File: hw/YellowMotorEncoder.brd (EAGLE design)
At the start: 35 x 22.2 mm, 20 parts, among them P1 M1

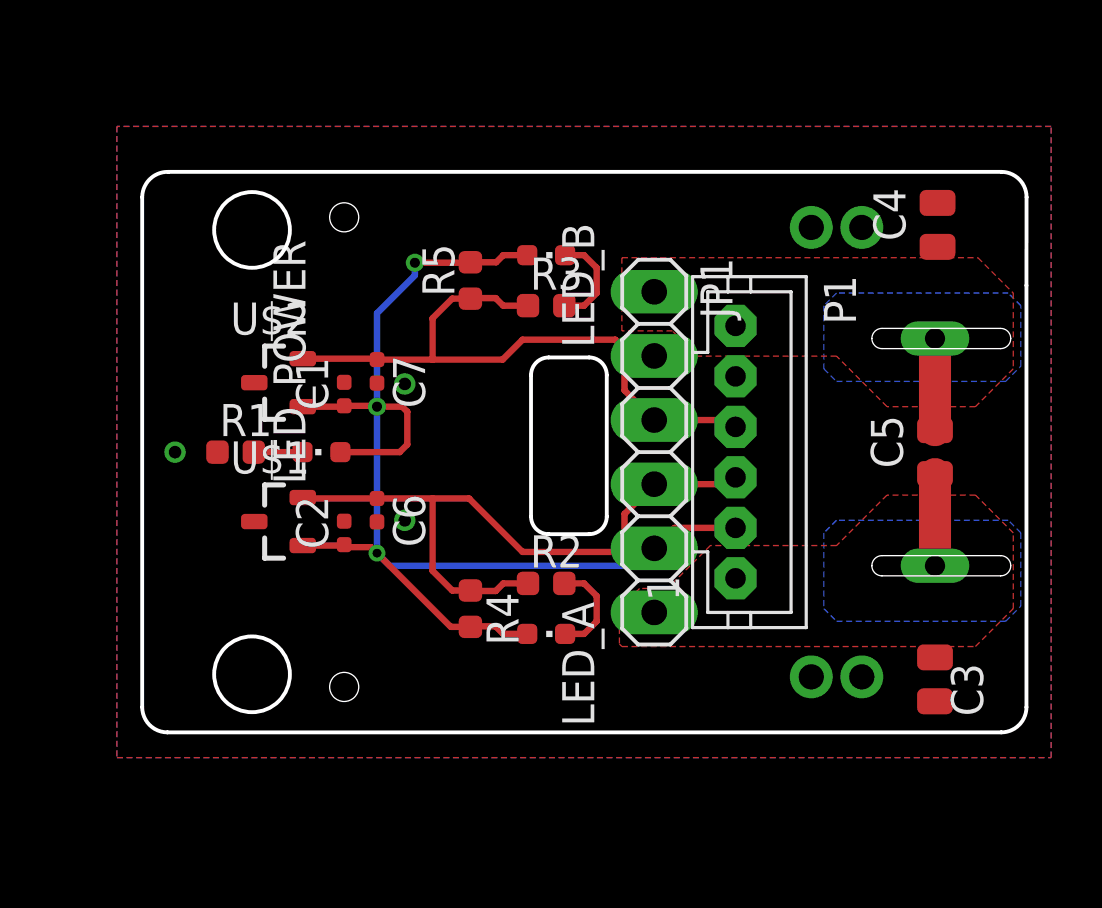
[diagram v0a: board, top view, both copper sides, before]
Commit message: FourProbes
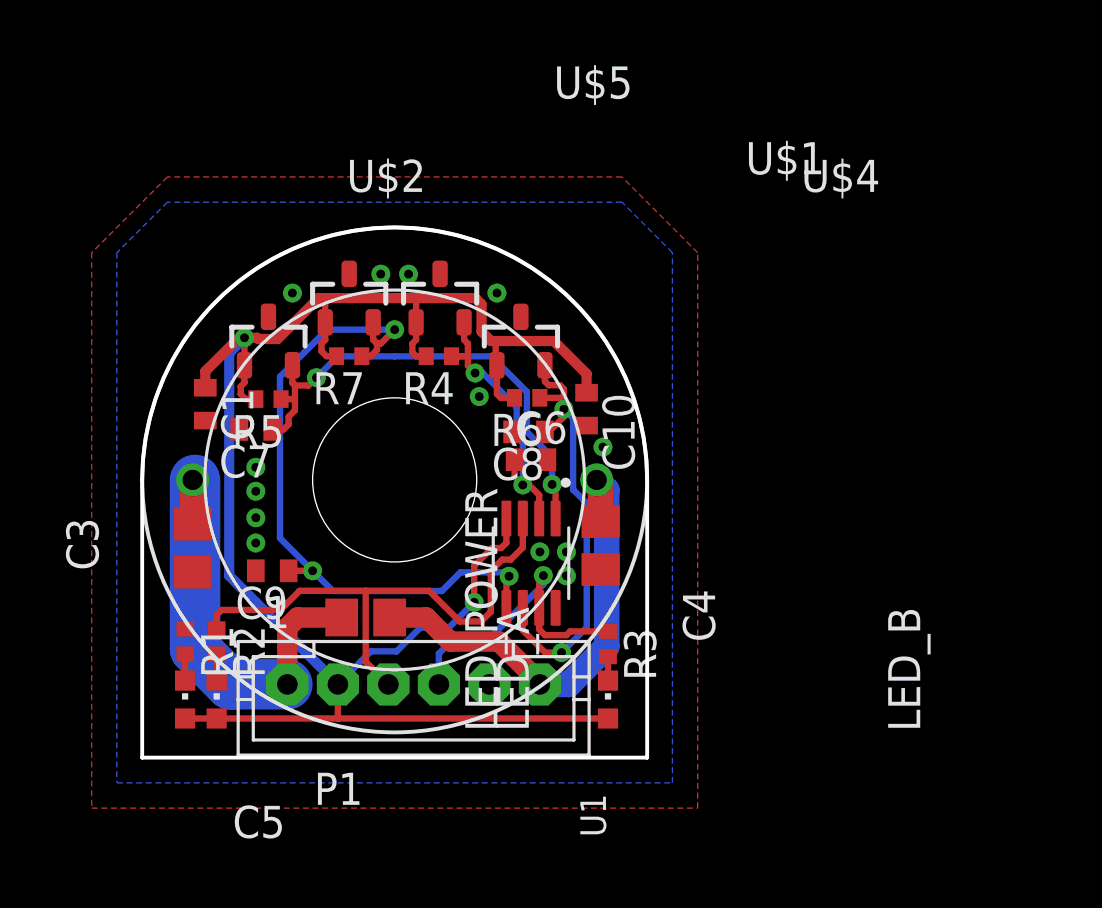
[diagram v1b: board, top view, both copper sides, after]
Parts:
- removed C2: 10n/50V, rcl:C0402
- removed JP1: (no value), pinhead:1X06
- removed U$3: YELLOW_MOTOR, motor:YELLOW_MOTOR
- added C10: 20n/50V, rcl:C0402
- added C8, C9: 18p/50V, rcl:C0402
- added M1: MOTOR, motor:OT-FK-130PH
- added R6, R7: 47k, rcl:R0402
- added U$4, U$5: MH253ESO, hall_sensor:SOT23
- added U1: SN74LVC2G86DCTR, SN74LVC2G86DCTR:SOP65P400X130-8N
- C1: value 10n/50V -> 20n/50V
- R1, R2, R3, R4, R5: device rcl:R0603 -> rcl:R0402
- moved C3 29.9 mm to (2.00, 7.30)
- moved C5 23.5 mm to (8.85, 4.55), turned to 0 degrees
- moved C4 18.4 mm to (18.1, 7.40), turned to 270 degrees
- moved LED_B 17.8 mm to (18.4, 1.30), turned to 0 degrees
- moved P1 15.7 mm to (10.8, 1.90), turned to 180 degrees
- moved R3 13.6 mm to (18.4, 3.50), turned to 270 degrees
- moved LED_A 13.3 mm to (2.95, 1.30), turned to 0 degrees
- moved R2 13.3 mm to (2.95, 3.60), turned to 270 degrees
- moved LED_POWER 11.2 mm to (1.70, 1.30)
- moved U$1 10.9 mm to (11.8, 17.2), turned to 270 degrees
- moved R4 10.1 mm to (11.8, 14.9), turned to 180 degrees
- moved R5 9.28 mm to (5.00, 13.2), turned to 180 degrees
- moved R1 7.76 mm to (1.70, 3.60), turned to 270 degrees
- moved C6 6.42 mm to (15.4, 10.8), turned to 0 degrees
- moved C1 5.51 mm to (2.50, 13.0), turned to 270 degrees
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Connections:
- new net A0: C8.1, R6.1, U$4.2, U1.6
- new net A1: C9.1, R7.1, U$5.2, U1.5
- new net B0: C6.1, R4.1, U$1.2, U1.2
- new net B1: C7.1, R5.1, U$2.2, U1.1
- net A: now also U1.3; no longer C6.1, JP1.4, R4.1, U$1.2
- net B: now also U1.7; no longer C7.1, JP1.3, R5.1, U$2.2
- net GND: now also C10.2, C8.2, C9.2, U$4.3, U$5.3, U1.8; no longer C2.2, JP1.2
- net M+: now also M1.P$1; no longer JP1.6, U$3.P$2
- net M-: now also M1.P$2; no longer JP1.1, U$3.P$1
- net VCC: now also C10.1, R6.2, R7.2, U$4.1, U$5.1, U1.4; no longer C2.1, JP1.5
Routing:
- net A1: track 0.00 -> 27.1 mm, vias 0 -> 3
- net VCC: track 50.4 -> 76.3 mm, vias 3 -> 2
- net B1: track 0.00 -> 19.5 mm, vias 0 -> 2
- net A0: track 0.00 -> 17.8 mm, vias 0 -> 2
- net M-: track 3.63 -> 18.8 mm
- net B: track 25.8 -> 11.9 mm, vias 0 -> 1
- net M+: track 3.63 -> 17.2 mm
- net B0: track 0.00 -> 11.1 mm, vias 0 -> 2
- net A: track 27.0 -> 21.0 mm
- net LED_TOP1: track 3.94 -> 0.95 mm
- net LED_SIDE1: track 3.94 -> 1.05 mm
- net LED_POWER: track 1.93 -> 1.05 mm
- removed copper zone on layer 1, net M+
- removed copper zone on layer 16, net M+
- removed copper zone on layer 1, net M-
- removed copper zone on layer 16, net M-
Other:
- board size 35 x 22.2 mm -> 20 x 21 mm
- board text removed: "A"
- board text removed: "B"
- board text removed: "JLCJLCJLCJLC"
- board text removed: "M- GND B A VCC M+"
- board text removed: "RB0003-YellowMotorEncoder"
- board text removed: "YellowMotorEncoder"
- board text removed: "github::roboticsbrno/"
- board text removed: "v1.2 CC BY-SA 4.0"

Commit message: ochrany
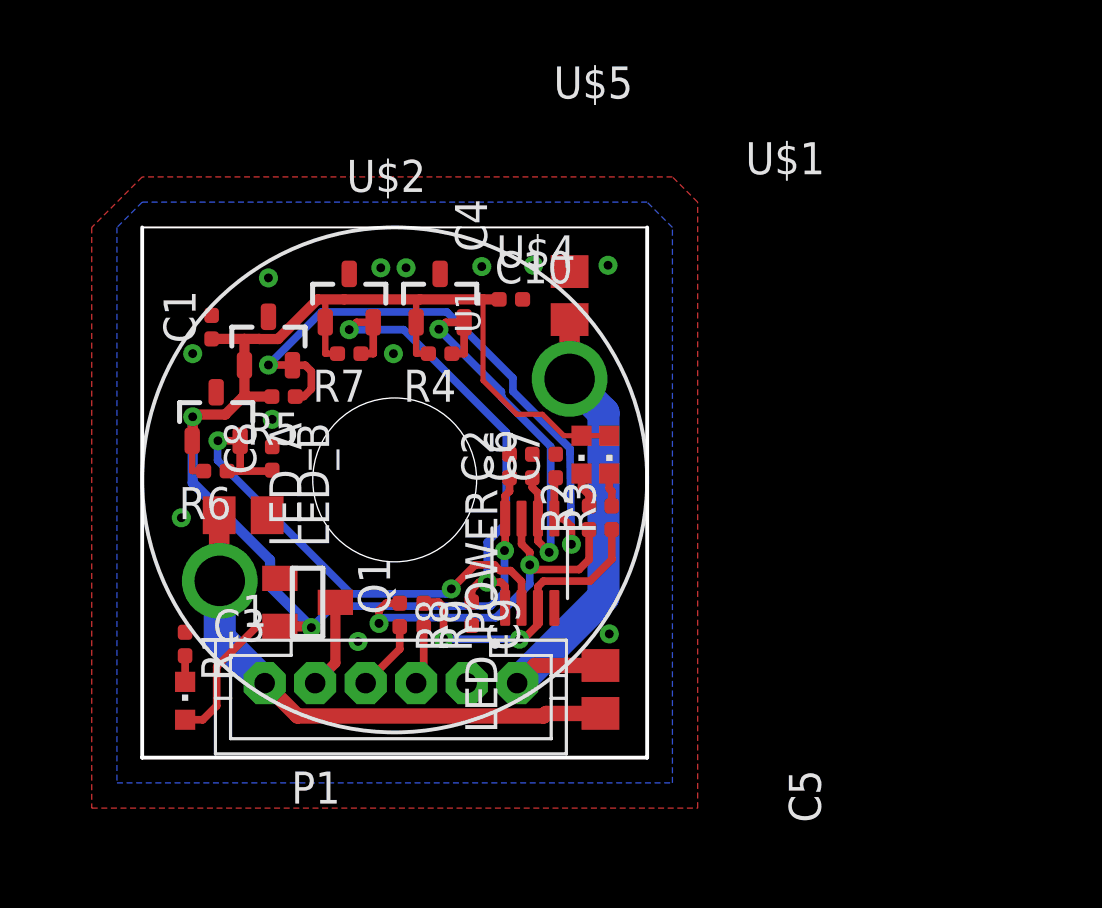
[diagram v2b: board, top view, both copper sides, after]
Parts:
- added C2: 20n/50V, rcl_upravena:C0402
- added Q1: FDN360P, transistor-power:SUPER-SOT3
- added R8, R9: 200, rcl_upravena:R0402
- C1, C10, C6, C7, C8, C9: device rcl:C0402 -> rcl_upravena:C0402
- M1: value MOTOR -> YELLOW_MOTORV2; device motor:OT-FK-130PH -> motor:YELLOW_MOTOR_V2
- R1, R2, R3, R4, R5, R6, R7: device rcl:R0402 -> rcl_upravena:R0402
- moved LED_A 17.4 mm to (17.4, 11.0), turned to 180 degrees
- moved R2 15.5 mm to (17.7, 8.50), turned to 90 degrees
- moved R6 12.7 mm to (2.90, 10.3)
- moved U$4 12.4 mm to (2.93, 12.5)
- moved C7 12.0 mm to (16.4, 10.6), turned to 90 degrees
- moved C8 10.2 mm to (5.15, 10.8), turned to 90 degrees
- moved C4 9.98 mm to (16.9, 17.3), turned to 90 degrees
- moved C5 9.73 mm to (18.1, 1.70), turned to 90 degrees
- moved LED_B 9.70 mm to (18.5, 11.0), turned to 180 degrees
- moved C9 8.08 mm to (13.1, 4.70), turned to 270 degrees
- moved C10 5.28 mm to (14.6, 17.1), turned to 0 degrees
- moved R3 5.00 mm to (18.6, 8.50), turned to 90 degrees
- moved C1 3.06 mm to (2.75, 16.1), turned to 90 degrees
- moved C3 2.39 mm to (4.00, 8.60), turned to 0 degrees
- moved P1 0.90 mm to (9.85, 1.95)
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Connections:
- new net !A: R2.1, R8.1, U1.7
- new net !B: R3.1, R9.1, U1.3
- new net N$1: P1.2, Q1.3
- net A: now also R8.2; no longer R2.1, U1.3
- net A0: now also U1.2; no longer U1.6
- net A1: now also U1.1; no longer U1.5
- net B: now also R9.2; no longer R3.1, U1.7
- net B0: now also U1.6; no longer U1.2
- net B1: now also U1.5; no longer U1.1
- net GND: now also C2.2, Q1.1, U1.4; no longer U1.8
- net VCC: now also C2.1, Q1.2, U1.8; no longer P1.2, U1.4
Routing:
- net A: track 21.0 -> 2.79 mm
- net !A: track 0.00 -> 14.6 mm, vias 0 -> 2
- net !B: track 0.00 -> 12.2 mm, vias 0 -> 2
- net VCC: track 76.3 -> 66.3 mm, vias 2 -> 3
- net B: track 11.9 -> 2.36 mm, vias 1 -> 0
- net A1: track 27.1 -> 19.8 mm, vias 3 -> 2
- net B1: track 19.5 -> 25.6 mm
- net B0: track 11.1 -> 16.8 mm
- net M+: track 17.2 -> 21.3 mm
- net N$1: track 0.00 -> 3.53 mm
- net A0: track 17.8 -> 20.7 mm
- net M-: track 18.8 -> 20.0 mm
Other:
- outline, holes or cut-outs redrawn
